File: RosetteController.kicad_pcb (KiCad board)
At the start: 4 copper layers, 52.9 x 45.4 mm, 89 parts, among them J1 284391-4, J2 284391-4, J3 284391-4, J4 284391-4, J5 284391-4, J6 284391-4, J7 Conn_ARM_SWD_TagConnect_TC2030, U1 PIC32CM1216MC00032, U10 PAC1720, U11 TPS1H000, U12 TPS1H000, U13 TLV6713, U2 MAX3222EIPWR, U3 TPSM33610S3Q, U4 LM4132AMF-2.0, U5 MAX11201, U6 TB67H450AFNG, U7 MX25L25645G, U8 MS860702BA01-50, U9 TLV6713

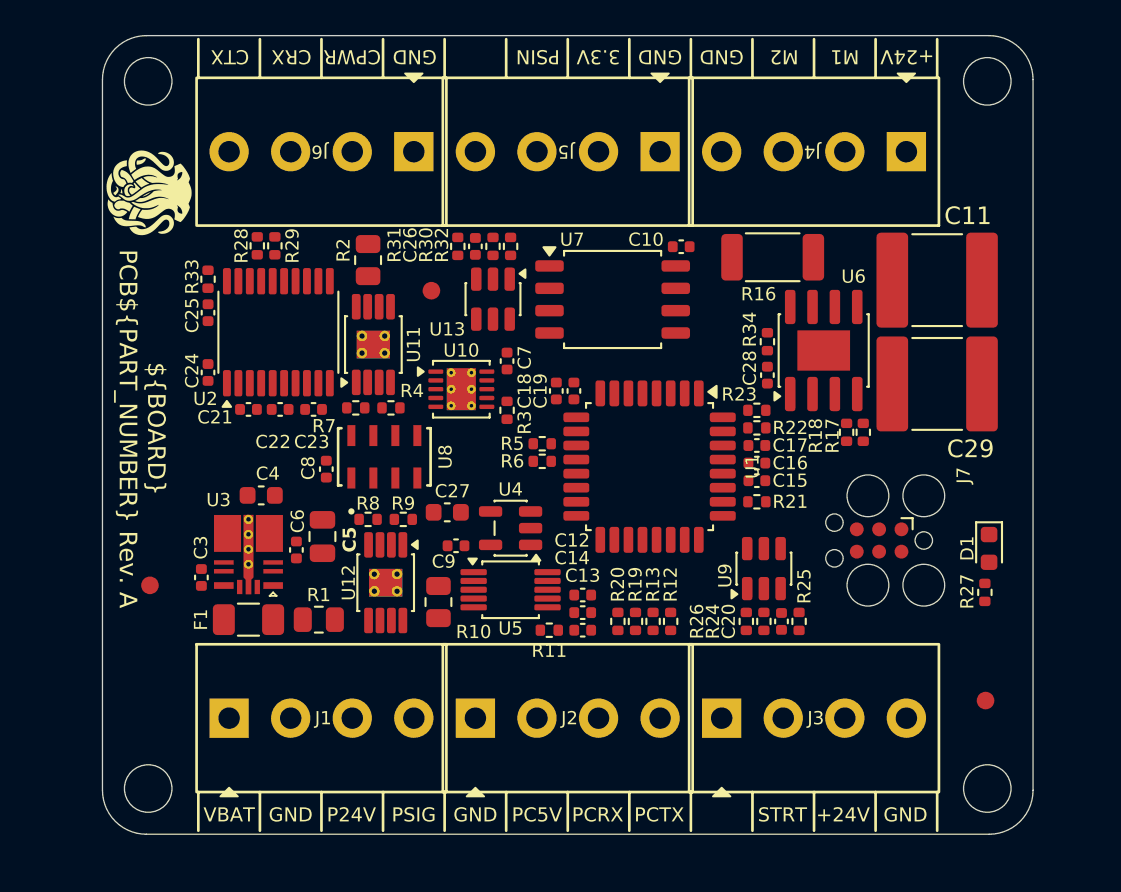
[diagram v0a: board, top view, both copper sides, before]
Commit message: Layout Complete
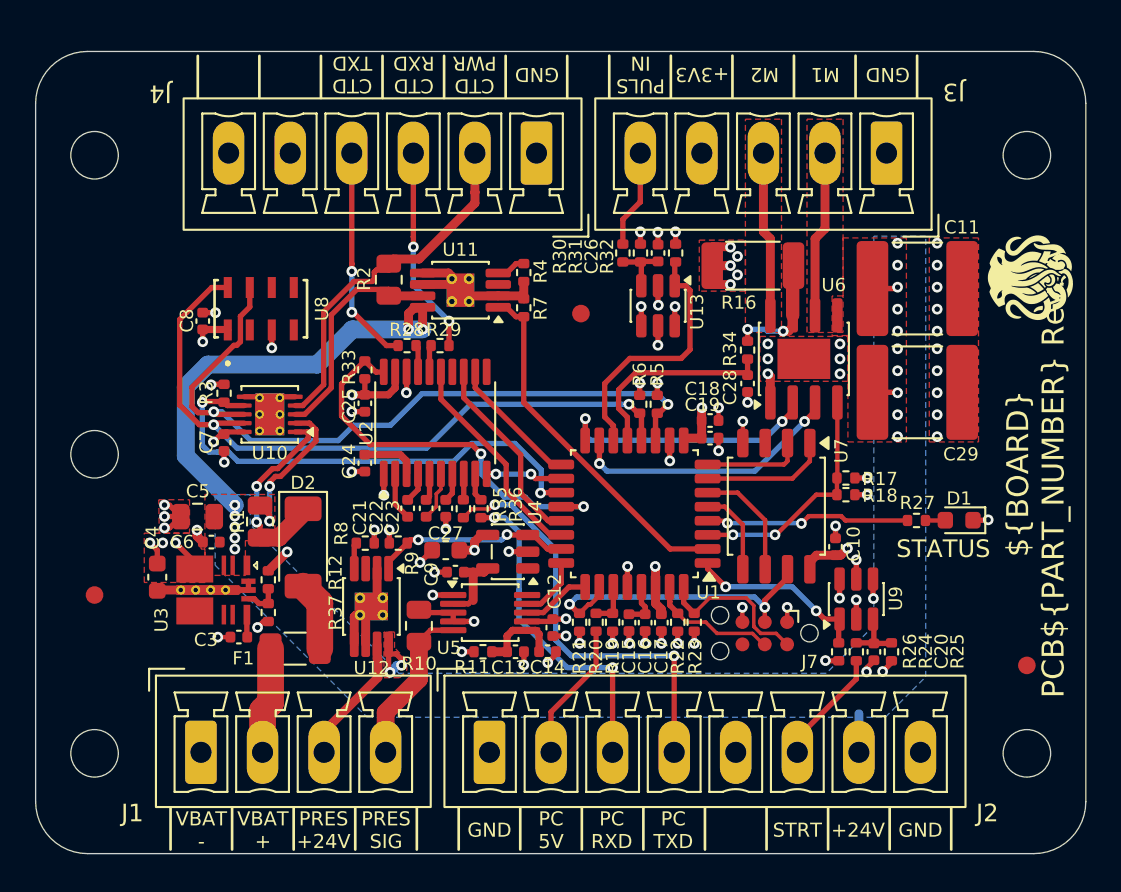
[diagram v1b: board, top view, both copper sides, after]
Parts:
- removed ? (x2): , 
- removed J5, J6: 284391-4, prj-footprints:CONN4_284391-4_TEC
- removed R13: 1k, Resistor_SMD:R_0402_1005Metric
- added D2: PMEG60T50ELPX, Diode_SMD:D_SOD-128, F.Cu at (184.2, 140.3)
- added FID2: Fiducial_1mm_Mask3mm, Fiducial:Fiducial_1mm_Mask3mm, F.Cu at (172.3, 143.0)
- added FID3: Fiducial_1mm_Mask3mm, Fiducial:Fiducial_1mm_Mask3mm, F.Cu at (200.0, 127.0)
- added R35: 330, Resistor_SMD:R_0402_1005Metric, F.Cu at (193.3, 138.1)
- added R36: 330, Resistor_SMD:R_0402_1005Metric, F.Cu at (194.3, 138.1)
- added R37: DNP, Resistor_SMD:R_0402_1005Metric, F.Cu at (182.2, 144.0)
- added REF**: MountingHole_2.7mm_M2.5, MountingHole:MountingHole_2.7mm_M2.5, F.Cu at (172.3, 118.0)
- J1: value 284391-4 -> 0395016004; footprint prj-footprints:CONN4_284391-4_TEC -> Connector_Phoenix_MC:PhoenixContact_MCV_1,5_4-G-3.5_1x04_P3.50mm_Vertical
- J2: value 284391-4 -> 0395016008; footprint prj-footprints:CONN4_284391-4_TEC -> Connector_Phoenix_MC:PhoenixContact_MCV_1,5_8-G-3.5_1x08_P3.50mm_Vertical
- J3: value 284391-4 -> 0395016005; footprint prj-footprints:CONN4_284391-4_TEC -> Connector_Phoenix_MC:PhoenixContact_MCV_1,5_5-G-3.5_1x05_P3.50mm_Vertical
- J4: value 284391-4 -> 0395016006; footprint prj-footprints:CONN4_284391-4_TEC -> Connector_Phoenix_MC:PhoenixContact_MCV_1,5_6-G-3.5_1x06_P3.50mm_Vertical
- J7: footprint Connector:Tag-Connect_TC2030-IDC-FP_2x03_P1.27mm_Vertical -> Connector:Tag-Connect_TC2030-IDC-NL_2x03_P1.27mm_Vertical
- R12: value 1k -> 0
- REF** (x4): value MountingHole_2.7mm_M2.5_ISO14580 -> MountingHole_2.7mm_M2.5; footprint MountingHole:MountingHole_2.7mm_M2.5_ISO14580 -> MountingHole:MountingHole_2.7mm_M2.5
- moved REF** 55.0 mm to (172.3, 135.0)
- moved G*** 50.3 mm to (225.6, 125.0), turned to 90 degrees
- moved REF** 50.1 mm to (225.3, 118.0)
- moved J3 33.5 mm to (217.4, 117.9), turned to 180 degrees
- moved R12 23.0 mm to (182.2, 142.1), turned to -90 degrees
- moved J4 21.0 mm to (197.5, 117.9)
- moved C10 19.2 mm to (214.5, 140.3), turned to 90 degrees
- moved C7 16.7 mm to (179.7, 134.3), turned to -90 degrees
- moved R3 16.1 mm to (179.7, 131.5), turned to -90 degrees
- moved U7 15.0 mm to (211.1, 137.9), turned to -90 degrees
- moved R23 12.6 mm to (206.4, 144.6), turned to 90 degrees
- moved R21 12.2 mm to (199.9, 144.6), turned to 90 degrees
- moved R22 11.9 mm to (205.5, 144.6), turned to 90 degrees
- moved C17 11.4 mm to (204.6, 144.6), turned to -90 degrees
- moved R7 11.1 mm to (196.8, 126.7), turned to 90 degrees
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- gave numbers to parts that had none: 1
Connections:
- F1 pad 2: Net-(U10-SENSE1+) -> Net-(D2-A)
- J1 pad 1: /VBATT+ -> GND
- J1 pad 2: GND -> /VBATT+
- J2 pad 3: /FTDI_RX -> /RS232_RX
- J2 pad 4: /FTDI_TX -> /RS232_TX
- J3 pad 1: unconnected-(J3-Pin_1-Pad1) -> GND
- J3 pad 2: /START_PLUG -> /MOTOR1
- J3 pad 3: +24V -> /MOTOR2
- J3 pad 4: GND -> +3.3V
- J4 pad 1: +24V -> GND
- J4 pad 2: /MOTOR1 -> /CTD_PWR
- J4 pad 3: /MOTOR2 -> /CTD_RX
- J4 pad 4: GND -> /CTD_TX
- R1 pad 1: Net-(U10-SENSE1+) -> Net-(D2-K)
- R12 pad 1: /FTDI_TX -> +3.3V
- R12 pad 2: /PC_TXD -> Net-(U3-FB)
- U1 pad 1: /PRES_ON -> /RUN_WAKE
- U1 pad 14: /PAC_ALERT -> /HALL_SENSOR
- U1 pad 19: /HALL_SENSOR -> /PAC_ALERT
- U1 pad 20: /RUN_WAKE -> /RS232_SHDN
- U1 pad 23: /LED -> /PRES_ON
- U1 pad 4: /RS232_SHDN -> /LED
- U10 pad 1: Net-(U10-SENSE1+) -> Net-(D2-K)
- U2 pad 10: unconnected-(U2-ROUT2-Pad10) -> /PC_RXD
- U2 pad 12: GND -> /PC_TXD
- U2 pad 8: unconnected-(U2-DOUT2-Pad8) -> Net-(U2-DOUT2)
- U2 pad 9: GND -> Net-(U2-RIN2)
- U3 pad 9: +3.3V -> Net-(U3-FB)
- U6 pad 9: (no net) -> GND
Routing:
- net GND: track 0.00 -> 72.1 mm, vias 0 -> 69
- net +24V: track 0.00 -> 44.0 mm, vias 0 -> 21
- net /SDA: track 0.00 -> 41.7 mm, vias 0 -> 2
- net /SCL: track 0.00 -> 40.1 mm, vias 0 -> 2
- net +3.3V: track 0.00 -> 36.6 mm, vias 0 -> 25
- net /PAC_ALERT: track 0.00 -> 28.2 mm, vias 0 -> 2
- net /RS232_TX: track 0.00 -> 25.2 mm, vias 0 -> 2
- net /RS232_SHDN: track 0.00 -> 22.9 mm, vias 0 -> 2
- net /CTD_PWR: track 0.00 -> 20.7 mm
- net /CTD_ON: track 0.00 -> 20.4 mm
- net /RS232_RX: track 0.00 -> 19.7 mm, vias 0 -> 2
- net /RESET: track 0.00 -> 17.9 mm, vias 0 -> 2
- net /MOTOR_IN1: track 0.00 -> 15.7 mm, vias 0 -> 2
- net /MOTOR_IN2: track 0.00 -> 15.3 mm, vias 0 -> 2
- net /HALL_SENSOR: track 0.00 -> 14.8 mm
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- added copper zone on B.Cu, net +24V
- added copper zone on F.Cu, net +24V
- added copper zone on F.Cu, net +3.3V
- added copper zone on F.Cu, net /MOTOR1
- added copper zone on F.Cu, net /MOTOR2
- added copper zone on F.Cu, net GND
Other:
- board size 52.9 x 45.4 mm -> 59.7 x 45.6 mm
- board text added: "+3V3"
- board text added: "CTD PWR"
- board text added: "CTD RXD"
- board text added: "CTD TXD"
- board text added: "PC 5V"
- board text added: "PC RXD"
- board text added: "PC TXD"
- board text added: "PRES +24V"
- board text added: "PRES SIG"
- board text added: "PULS IN"
- board text added: "STATUS"
- board text added: "VBAT +"
- board text added: "VBAT -"
- board text removed: "3.3V"
- board text removed: "CPWR"
- board text removed: "CRX"
- board text removed: "CTX"
- board text removed: "P24V"
- board text removed: "PC5V"
- board text removed: "PCRX"
- board text removed: "PCTX"
- board text removed: "PSIG"
- board text removed: "PSIN"
- board text removed: "VBAT"
